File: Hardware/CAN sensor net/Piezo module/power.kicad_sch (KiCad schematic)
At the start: 12 parts, among them U4 L78L05_SOT89, U5 LD3985M33R_SOT23, U6 L79L05_SOT89

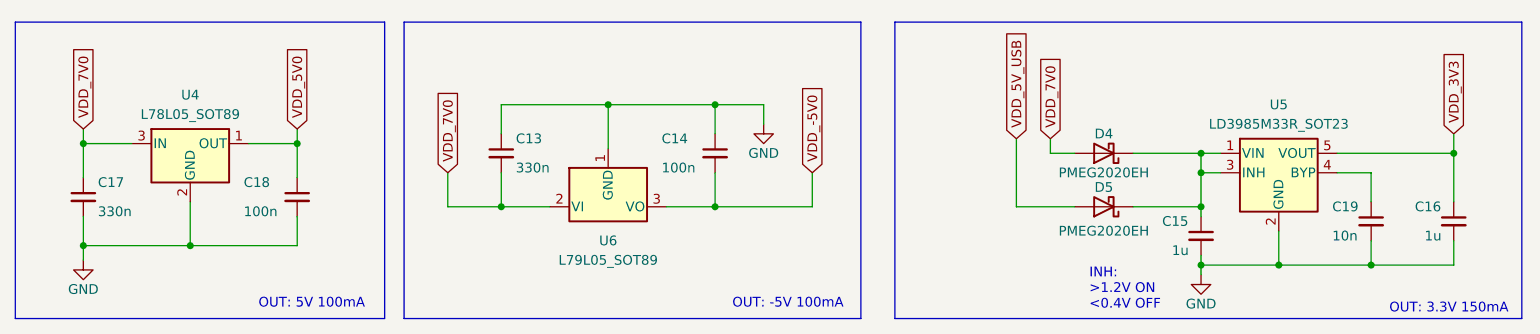
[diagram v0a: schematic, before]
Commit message: Minor fixes
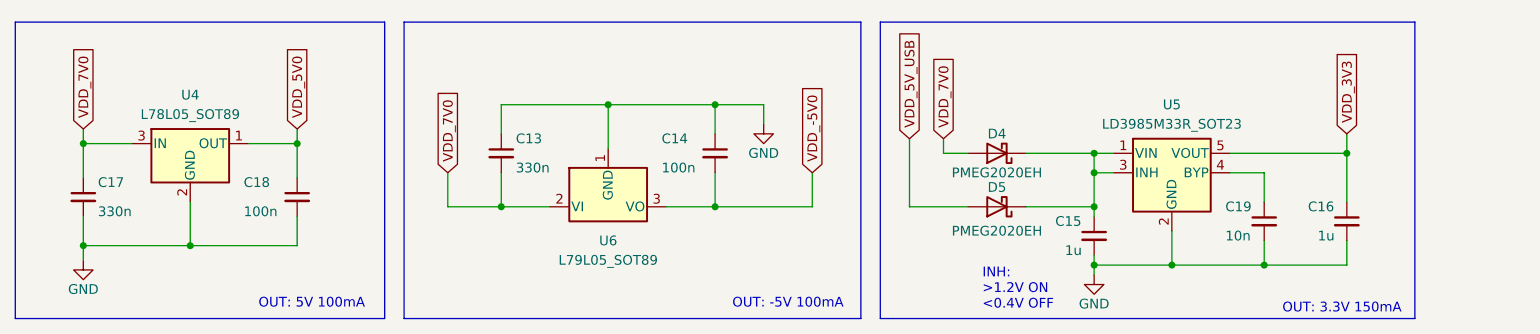
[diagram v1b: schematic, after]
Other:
- moved on the sheet: C15, C16, C19, D4, D5, U5
